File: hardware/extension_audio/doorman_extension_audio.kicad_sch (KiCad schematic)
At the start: 54 parts, among them J1 Output, J2 GPIO, J3 Input, J4 Extension Board Connector, U2 ES8311

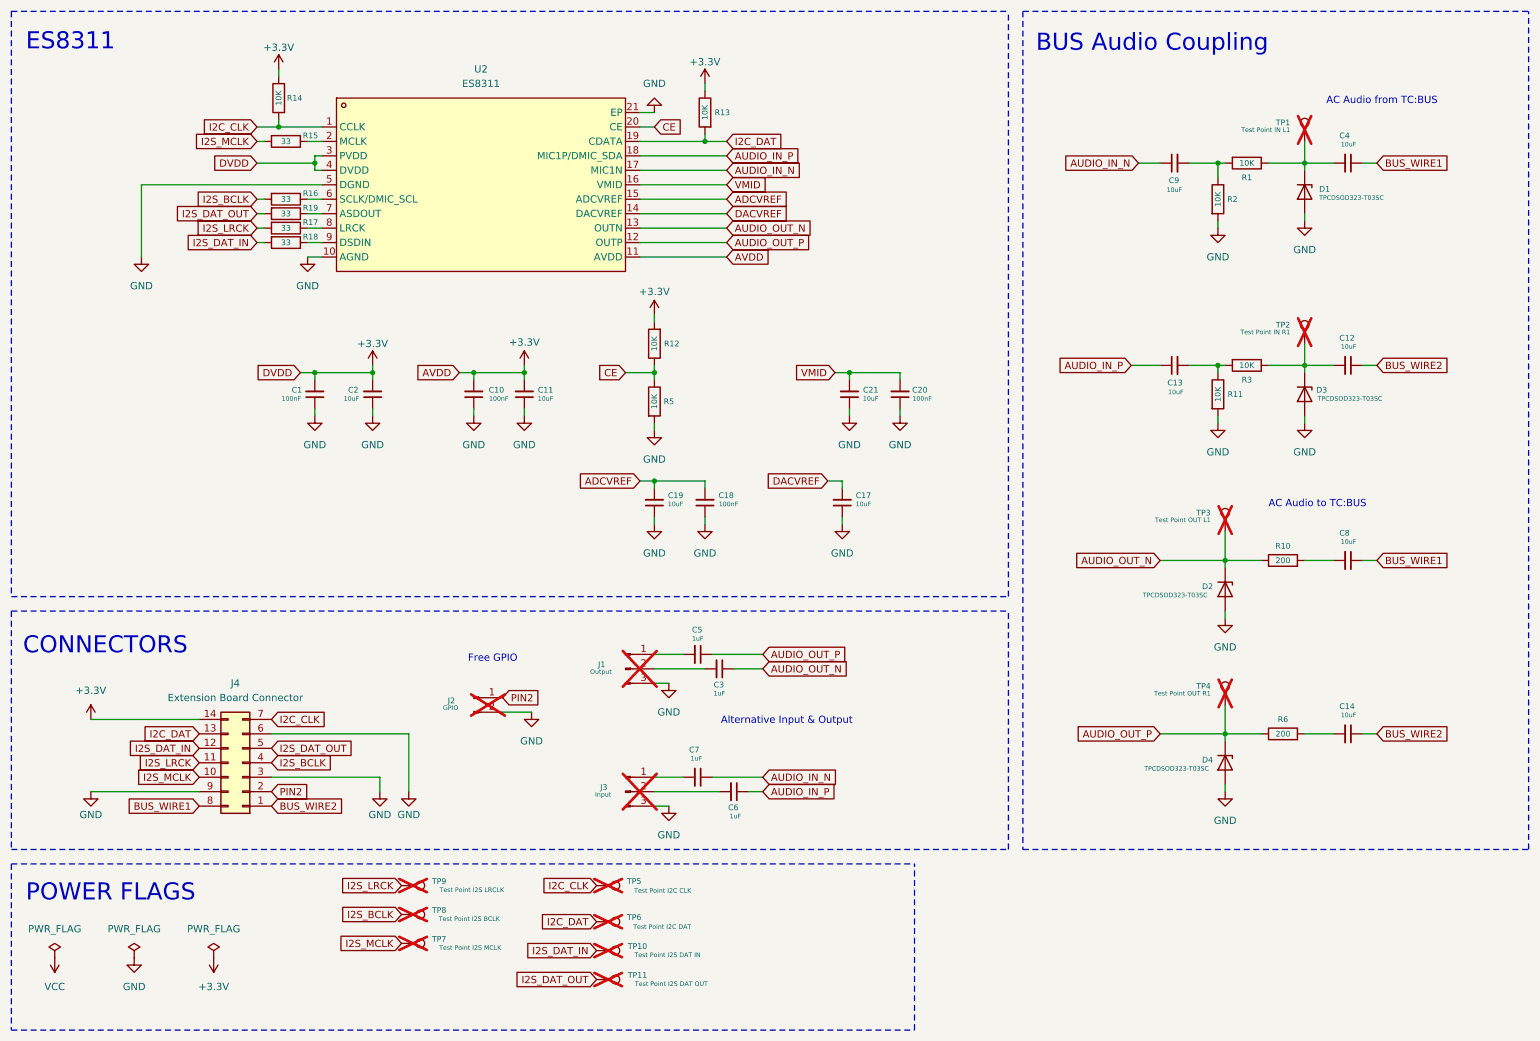
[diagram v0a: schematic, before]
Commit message: WIP
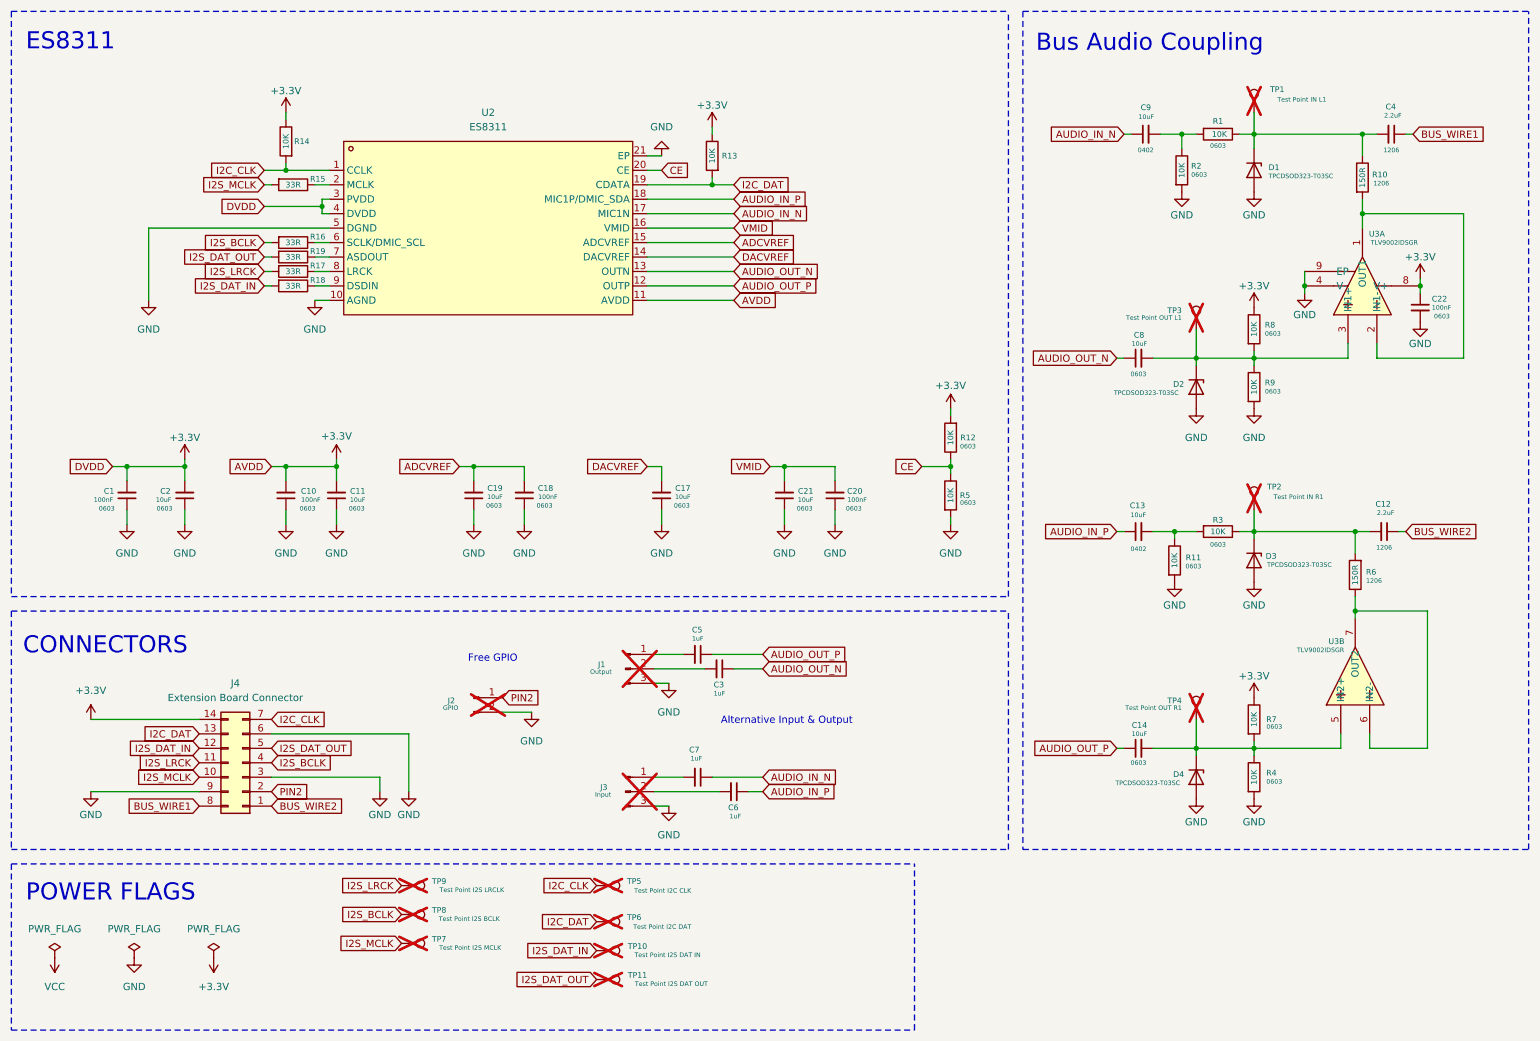
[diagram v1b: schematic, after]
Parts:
- added C22: 100nF, Capacitor_SMD:C_0603_1608Metric, symbol Device:C_Small
- added R4, R7, R8, R9: 10K, Resistor_SMD:R_0603_1608Metric, symbol Device:R
- added U3: TLV9002IDSGR, Doorman:WSON-8_L2.0-W2.0-P0.65-BL-EP, symbol easyeda2kicad:TLV9002IDSGR
- C12, C4: value 10uF -> 2.2uF; LCSC C89632 -> C50254; MPN CL31B106KBHNNNE -> CL31B225KBHNNNE
- C14, C8: footprint Capacitor_SMD:C_1206_3216Metric -> Capacitor_SMD:C_0603_1608Metric; LCSC C89632 -> C2959727; MPN CL31B106KBHNNNE -> GRM188Z71A106KA73D; Package 1206 -> 0603
- J2: now in the parts list
- R10, R6: value 200 -> 150R; LCSC C18002 -> C17917; MPN 1206W4F2000T5E -> 1206W4F1500T5E
- R15, R16, R17, R18, R19: value 33 -> 33R
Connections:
- net +3.3V: now also C22.1, R7.1, R8.1, U3.8 (V+)
- net AUDIO_OUT_N: now also C8.1; no longer D2.1 (K), R10.1, TP3.1
- net AUDIO_OUT_P: now also C14.1; no longer D4.1 (K), R6.1, TP4.1
- net BUS_WIRE1: no longer C8.1
- net BUS_WIRE2: no longer C14.1
- net GND: now also C22.2, R4.2, R9.2, U3.4 (V-), U3.9 (EP)
- net at C4.2, D1.1 (K), R1.1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: now also R10.1
- net at C12.2, D3.1 (K), R3.1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: now also R6.2
- net at C14.2: now also D4.1 (K), TP4.1, R4.1, R7.2, U3.5 (IN2+); no longer R6.2
- net at C8.2: now also D2.1 (K), TP3.1, R8.2, R9.1, U3.3 (IN1+); no longer R10.2
- new net: R10.2, U3.1 (OUT1), U3.2 (IN1-)
- new net: R6.1, U3.6 (IN2-), U3.7 (OUT2)
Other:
- note added: "Bus Audio Coupling"
- note removed: "AC Audio from TC:BUS"
- note removed: "AC Audio to TC:BUS"
- note removed: "BUS Audio Coupling"
- moved on the sheet: C1, C10, C11, C12, C13, C17, C18, C19, C2, C20, C21, C4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
